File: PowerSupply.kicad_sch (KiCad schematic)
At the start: 8 parts, among them U301 TPSM33625

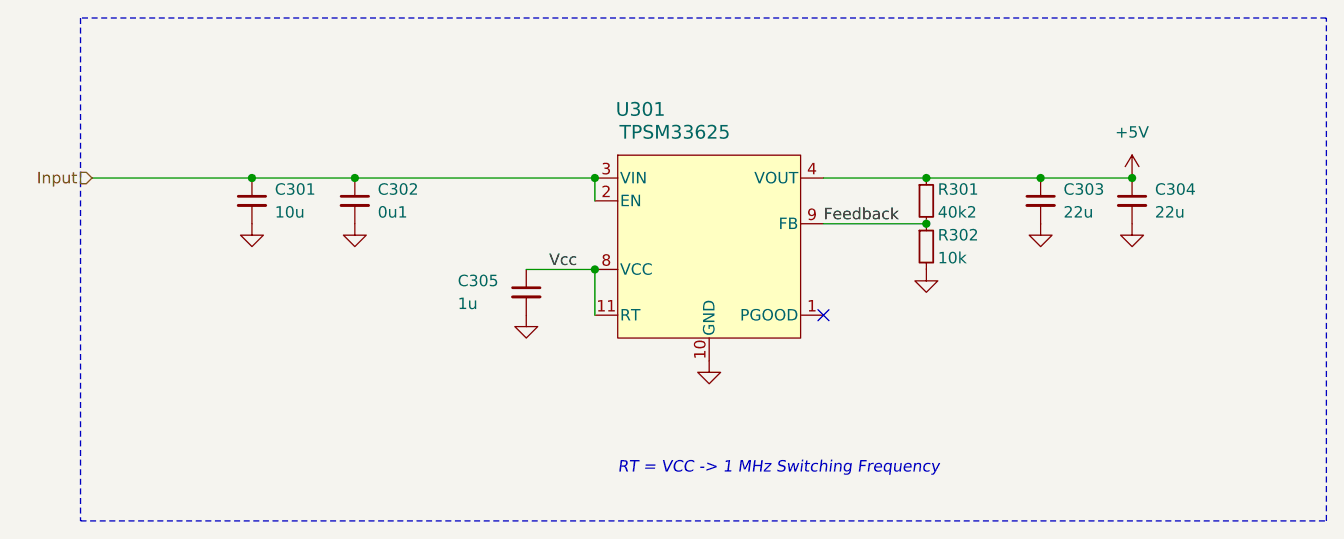
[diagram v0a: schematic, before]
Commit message: Update parts
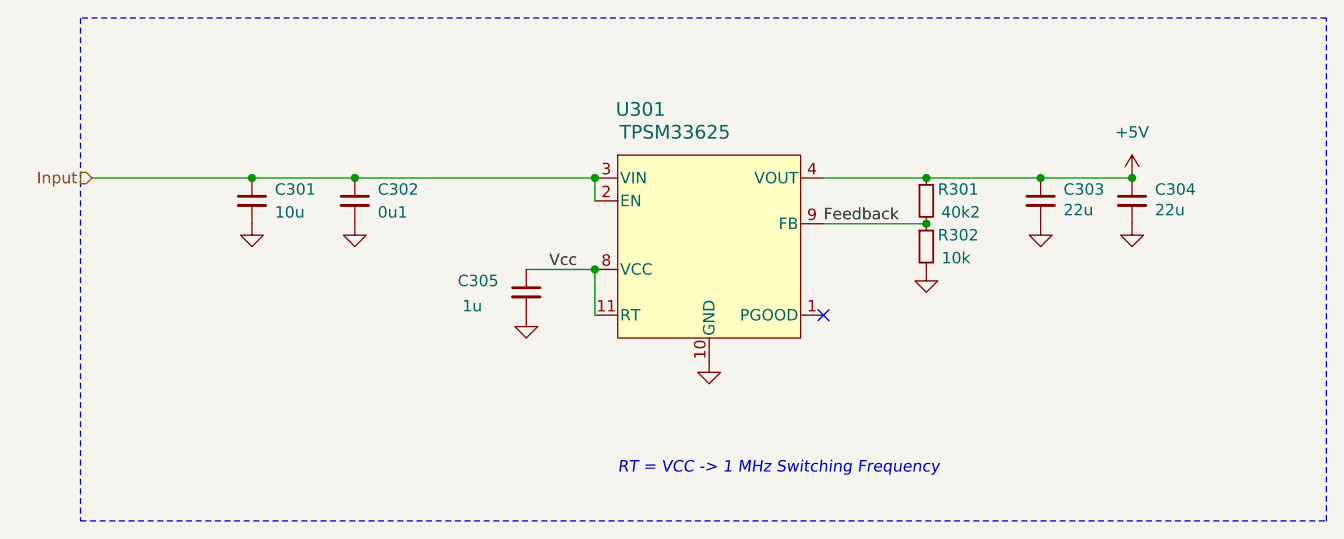
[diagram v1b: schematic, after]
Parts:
- C301: footprint Capacitor_SMD:C_1210_3225Metric -> V2_Capacitor_SMD:C_1210; symbol Device:C_Small -> V2_Device:C_1210_10u; Manufacturer (none) -> TDK; Mouser (none) -> 810-CNA6P1X7R1H106K2; Product (none) -> CNA6P1X7R1H106K250AE; Rating (none) -> 50V; Voltage (none) -> 50V
- C302: footprint Capacitor_SMD:C_0603_1608Metric -> V2_Capacitor_SMD:C_0603; symbol Device:C_Small -> V2_Device:C_0603_0u1; Manufacturer (none) -> TDK; Mouser (none) -> 810-CGA3E2X7R1H104MA; Product (none) -> CGA3E2X7R1H104M080AA
- C303, C304: footprint Capacitor_SMD:C_1210_3225Metric -> V2_Capacitor_SMD:C_1210; symbol Device:C_Small -> V2_Device:C_1210_22u; Manufacturer (none) -> TDK; Mouser (none) -> 810-CGA6P3X7R1E226M5; Product (none) -> CGA6P3X7R1E226M250AE; Rating (none) -> 25V; Voltage (none) -> 25V
- C305: footprint Capacitor_SMD:C_0603_1608Metric -> V2_Capacitor_SMD:C_0603; symbol Device:C_Small -> V2_Device:C_0603_1u; Manufacturer (none) -> YAGEO; Mouser (none) -> 603-CC603KRX7R9BB105; Product (none) -> CC0603KRX7R9BB105
- R301: footprint Resistor_SMD:R_0603_1608Metric -> V2_Resistor_SMD:R_0603; symbol Device:R_Small -> V2_Device:R_0603_40k2; Manufacturer (none) -> Vishay; Mouser (none) -> 71-RCS060340K2FKEA; Product (none) -> RCS060340K2FKEA; Rating (none) -> 500mW
- R302: footprint Resistor_SMD:R_0603_1608Metric -> V2_Resistor_SMD:R_0603; symbol Device:R_Small -> V2_Device:R_0603_10k; Manufacturer (none) -> Vishay; Mouser (none) -> 71-CRCW060310K0FKEAC; Product (none) -> CRCW060310K0FKEAC; Rating (none) -> 100mW
- U301: Manufacturer (none) -> Texas Instruments; Mouser (none) -> 595-TPSM33625RDNR; Product (none) -> TPSM33625RDNR

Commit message: Update library
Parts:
- C301: Voltage 50V -> (none)
- C302: Rating (none) -> 50V
- C303, C304: Voltage 25V -> (none)
- C305: Manufacturer YAGEO -> TDK; Mouser 603-CC603KRX7R9BB105 -> 810-CGA3E3X7R1H105K0; Product CC0603KRX7R9BB105 -> CGA3E3X7R1H105K080AB; Rating (none) -> 50V
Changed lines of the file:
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@@
-			)
-		)
-		(property "Sim.Pin" ""
-			(at 148.59 102.87 0)
-			(effects
-				(font
-					(size 1.27 1.27)
-				)
-				(hide yes)
 			)
 		)
@@
 			)
 		)
-		(property "Sim.Pin" ""
-			(at 109.22 97.79 0)
-			(effects
-				(font
-					(size 1.27 1.27)
-				)
-				(hide yes)
-			)
-		)
 		(property "Manufacturer" "TDK"
 			(at 109.22 113.03 0)
@@
 			)
 		)
+		(property "Rating" "50V"
+			(at 109.22 120.65 0)
+			(effects
+				(font
+					(size 1.27 1.27)
+				)
+				(hide yes)
+			)
+		)
 		(pin "1"
 		)
@@
 			)
 		)
-		(property "Sim.Pin" ""
-			(at 195.58 97.79 0)
-			(effects
-				(font
-					(size 1.27 1.27)
-				)
-				(hide yes)
-			)
-		)
 		(property "Product" "CGA6P3X7R1E226M250AE"
 			(at 195.58 115.57 0)
@@
 			)
 		)
-		(property "Voltage" "25V"
-			(at 195.58 118.11 0)
-			(effects
-				(font
-					(size 1.27 1.27)
-				)
-				(hide yes)
-			)
-		)
 		(pin "1"
 		)
@@
 			)
 		)
-		(property "Sim.Pin" ""
-			(at 172.72 97.79 0)
-			(effects
-				(font
-					(size 1.27 1.27)
-				)
-				(hide yes)
-			)
-		)
 		(property "Rating" "500mW"
 			(at 172.72 118.11 0)
@@
 			)
 		)
-		(property "Description" "Power symbol creates a global label with name \"GND\" , ground"
+		(property "Description" ""
 			(at 185.42 100.33 0)
 			(effects
@@
 			)
 		)
-		(property "Description" "Power symbol creates a global label with name \"GND\" , ground"
+		(property "Description" ""
 			(at 195.58 100.33 0)
 			(effects
@@
 			)
 		)
-		(property "Description" "Power symbol creates a global label with name \"+5V\""
+		(property "Description" ""
 			(at 195.58 95.25 0)
 			(effects
@@
 			)
 		)
-		(property "Description" "Power symbol creates a global label with name \"GND\" , ground"
+		(property "Description" ""
 			(at 97.79 100.33 0)
 			(effects
@@
 			)
 		)
-		(property "Description" "Power symbol creates a global label with name \"GND\" , ground"
+		(property "Description" ""
 			(at 172.72 105.41 0)
 			(effects
@@
 			)
 		)
-		(property "Description" "Power symbol creates a global label with name \"GND\" , ground"
+		(property "Description" ""
 			(at 109.22 100.33 0)
 			(effects
@@
 			)
 		)
-		(property "Mouser" "603-CC603KRX7R9BB105"
+		(property "Mouser" "810-CGA3E3X7R1H105K0"
 			(at 128.27 125.222 0)
 			(effects
@@
 			)
 		)
-		(property "Sim.Pin" ""
-			(at 128.27 107.95 0)
-			(effects
-				(font
-					(size 1.27 1.27)
-				)
-				(hide yes)
-			)
-		)
-		(property "Product" "CC0603KRX7R9BB105"
+		(property "Product" "CGA3E3X7R1H105K080AB"
 			(at 128.27 125.73 0)
 			(effects
@@
 			)
 		)
-		(property "Manufacturer" "YAGEO"
+		(property "Manufacturer" "TDK"
 			(at 128.27 123.19 0)
+			(effects
+				(font
+					(size 1.27 1.27)
+				)
+				(hide yes)
+			)
+		)
+		(property "Rating" "50V"
+			(at 128.27 130.81 0)
 			(effects
 				(font
@@
 			)
 		)
-		(property "Sim.Pin" ""
-			(at 185.42 97.79 0)
-			(effects
-				(font
-					(size 1.27 1.27)
-				)
-				(hide yes)
-			)
-		)
 		(property "Product" "CGA6P3X7R1E226M250AE"
 			(at 185.42 115.57 0)
@@
 			)
 		)
-		(property "Voltage" "25V"
-			(at 185.42 118.11 0)
-			(effects
-				(font
-					(size 1.27 1.27)
-				)
-				(hide yes)
-			)
-		)
 		(pin "1"
 		)
@@
 			)
 		)
-		(property "Description" "Power symbol creates a global label with name \"GND\" , ground"
+		(property "Description" ""
 			(at 128.27 110.49 0)
 			(effects
@@
 			)
 		)
-		(property "Sim.Pin" ""
-			(at 172.72 102.87 0)
-			(effects
-				(font
-					(size 1.27 1.27)
-				)
-				(hide yes)
-			)
-		)
 		(property "Product" "CRCW060310K0FKEAC"
 			(at 172.72 120.65 0)
@@
 			)
 		)
-		(property "Description" "Power symbol creates a global label with name \"GND\" , ground"
+		(property "Description" ""
 			(at 148.59 115.57 0)
 			(effects
@@
 			)
 		)
-		(property "Sim.Pin" ""
-			(at 97.79 97.79 0)
-			(effects
-				(font
-					(size 1.27 1.27)
-				)
-				(hide yes)
-			)
-		)
 		(property "Product" "CNA6P1X7R1H106K250AE"
 			(at 97.79 115.57 0)
@@
 			(effects
 				(font
-					(size 1.27 1.27)
-				)
-				(hide yes)
-			)
-		)
-		(property "Voltage" "50V"
-			(at 97.79 118.11 0)
-			(effects
-				(font
